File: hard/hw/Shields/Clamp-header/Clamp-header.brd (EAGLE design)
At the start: 91.4 x 59.5 mm, 26 parts, among them J1 6p-2.54-90d, J10 6p-SMD-2.54, J11 6p-smd-2.54-90d, J12 6p-2.54-90d, J13 6p-2.54-90d, J14 6p-SMD-2.54, J2 6p-smd-2.54-90d, J3 6p-smd-2.54-90d, J4 6p-SMD-2.54, J5 6p-2.54-90d, J6 6p-2.54-90d, J7 6p-smd-2.54-90d, J8 6p-2.54-90d, J9 6p-2.54-90d

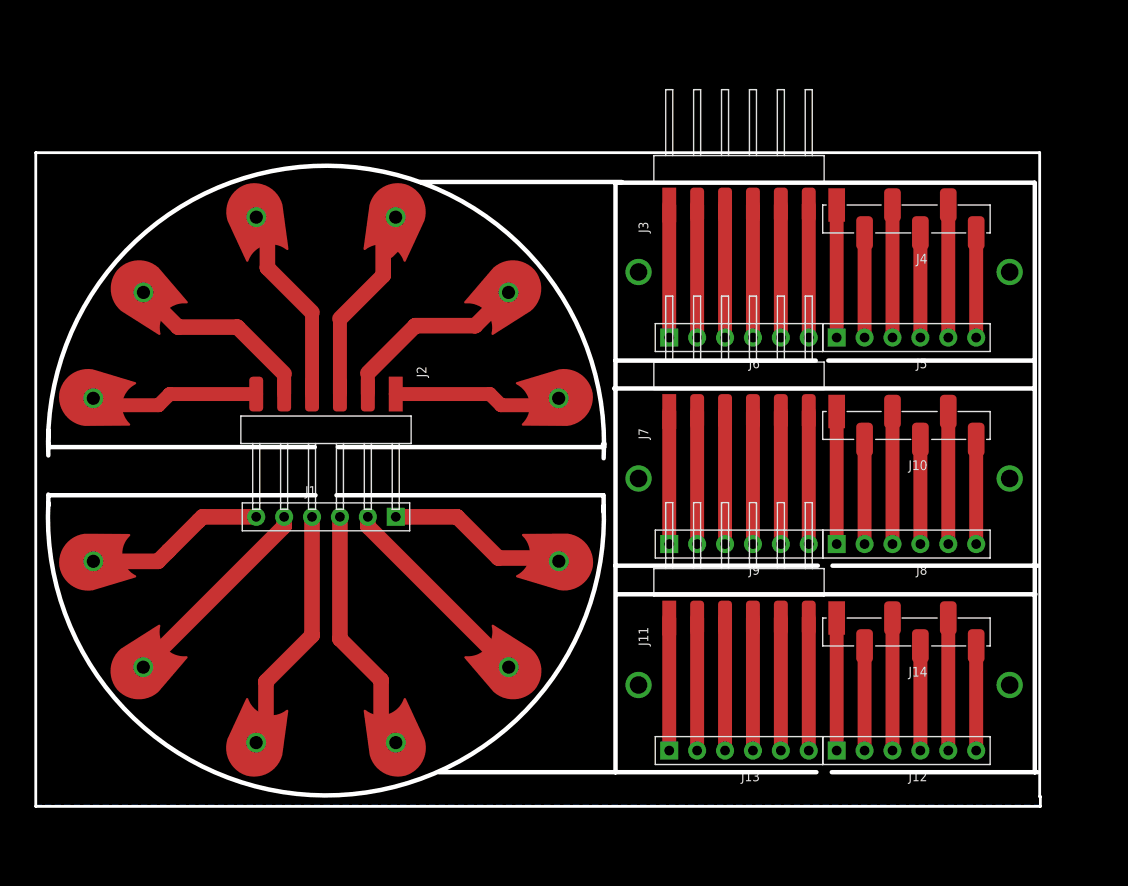
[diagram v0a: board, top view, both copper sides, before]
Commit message: Terminado Shield
by Ruben
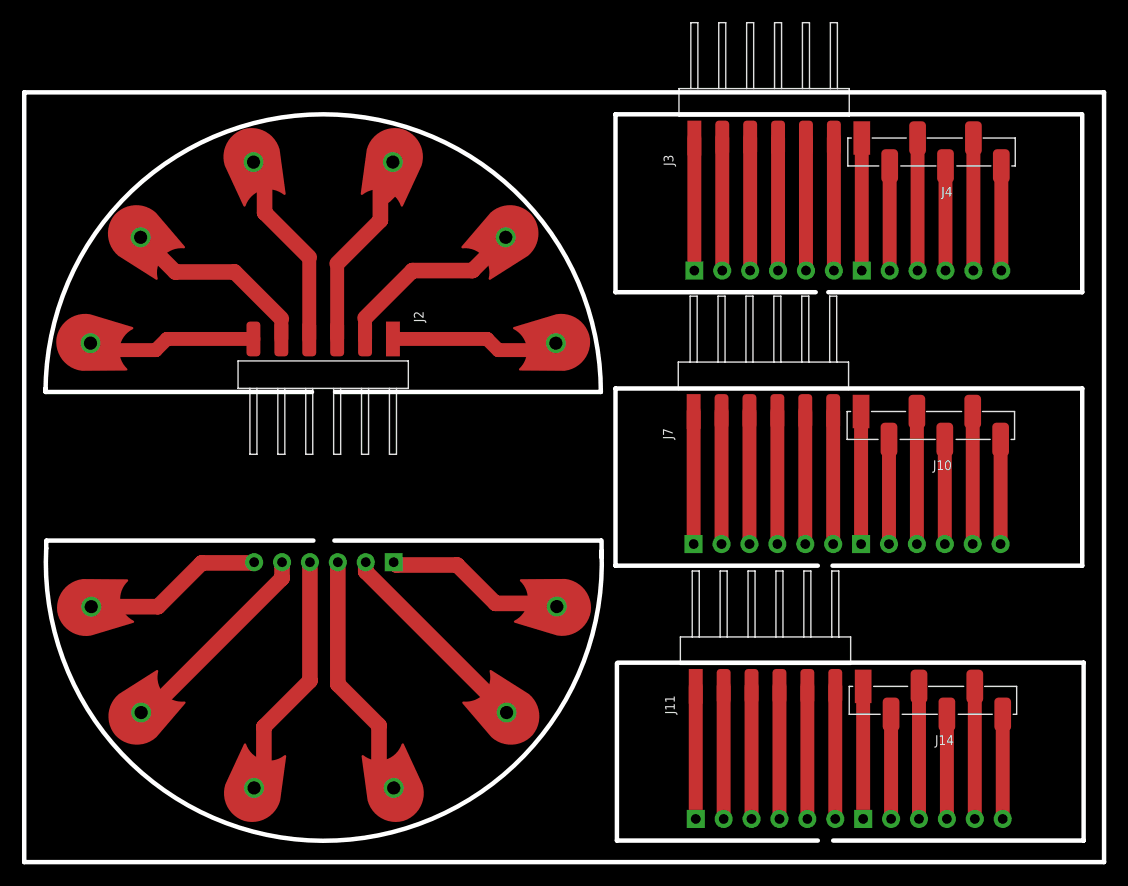
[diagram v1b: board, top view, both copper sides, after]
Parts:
- moved J14 6.67 mm to (83.6, 11.5)
- moved J12 6.67 mm to (83.6, 0.70), flipped to the bottom, turned to 270 degrees
- moved J13 6.67 mm to (68.3, 0.70), flipped to the bottom, turned to 270 degrees
- moved J11 6.67 mm to (68.3, 12.8)
- moved J3 6.51 mm to (68.2, 62.7)
- moved J6 6.51 mm to (68.2, 50.6), flipped to the bottom, turned to 270 degrees
- moved J4 6.51 mm to (83.4, 61.4)
- moved J5 6.51 mm to (83.4, 50.6), flipped to the bottom, turned to 270 degrees
- moved J2 5.02 mm to (28.1, 44.4)
- moved U$1 5.02 mm to (21.7, 60.5)
- moved U$2 5.02 mm to (6.86, 44.0)
- moved U$3 5.02 mm to (49.3, 44.0)
- moved U$5 5.02 mm to (11.4, 53.7)
- moved U$6 5.02 mm to (44.7, 53.7)
- moved U$7 5.02 mm to (34.4, 60.5)
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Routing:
- removed copper zone on layer 16, net GND
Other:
- board size 91.4 x 59.5 mm -> 98.3 x 70.1 mm
